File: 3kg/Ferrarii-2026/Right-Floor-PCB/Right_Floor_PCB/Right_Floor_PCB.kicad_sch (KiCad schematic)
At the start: 12 parts

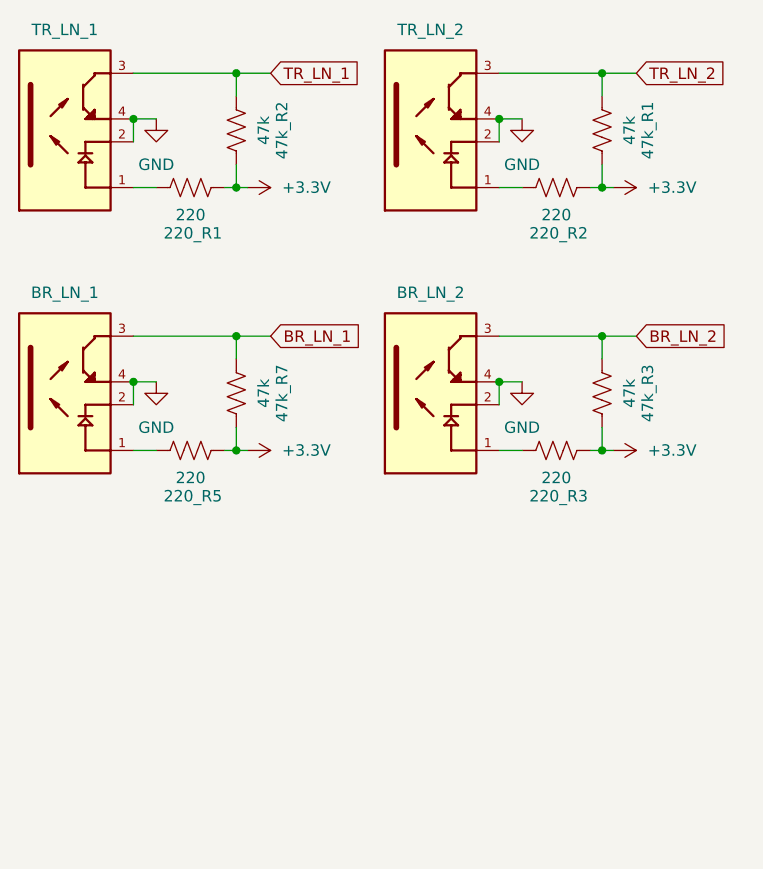
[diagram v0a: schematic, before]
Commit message: implemented entire floor pcb
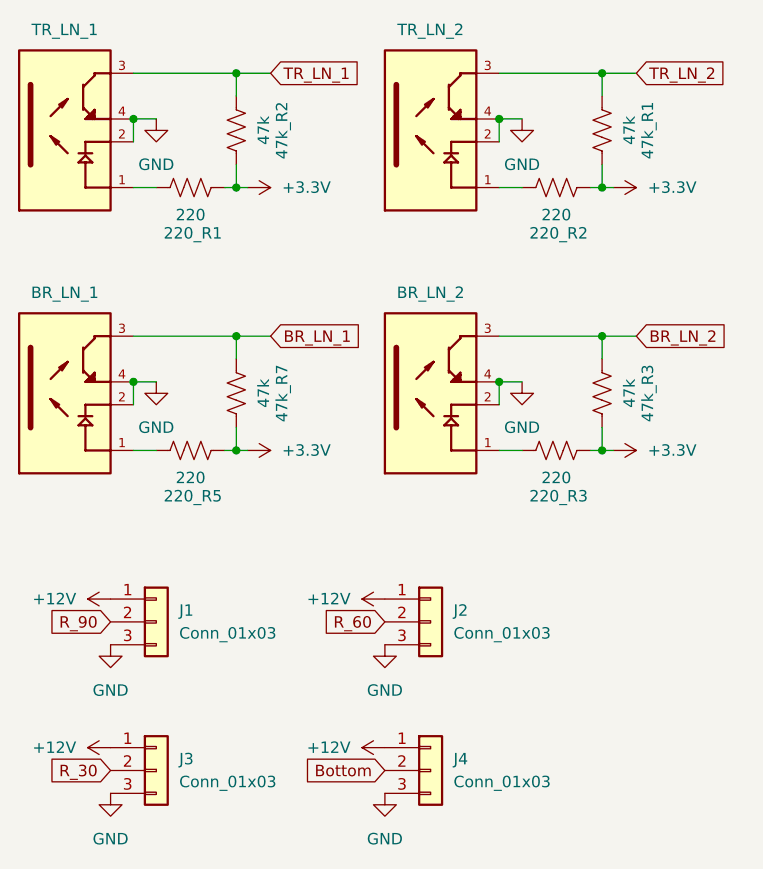
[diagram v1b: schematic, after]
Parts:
- added J1, J2, J3, J4: Conn_01x03, symbol Connector_Generic:Conn_01x03
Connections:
- net GND: now also J1.3 (Pin_3), J2.3 (Pin_3), J3.3 (Pin_3), J4.3 (Pin_3)
- new net +12V: J1.1 (Pin_1), J2.1 (Pin_1), J3.1 (Pin_1), J4.1 (Pin_1)
- new net Bottom: J4.2 (Pin_2)
- new net R_30: J3.2 (Pin_2)
- new net R_60: J2.2 (Pin_2)
- new net R_90: J1.2 (Pin_2)
